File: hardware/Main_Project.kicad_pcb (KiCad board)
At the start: 2 copper layers, 246.8 x 135.9 mm, 64 parts, among them J1 Motors_R, J10 BBBBBBBONUSROUND, J11 Power_Distro, J12 Power_Distro, J13 Power_Distro, J14 Power_Distro, J15 Color_Sensor, J16 Color_Sensor, J2 Motors_L, J3 Power_Outputs, J4 Motor_Control, J5 Motor_Power, J6 Motor_Power, J7 Motor_Control, J8 Color_Sensor, J9 Magnet?, U1 L7805, U2 L298N

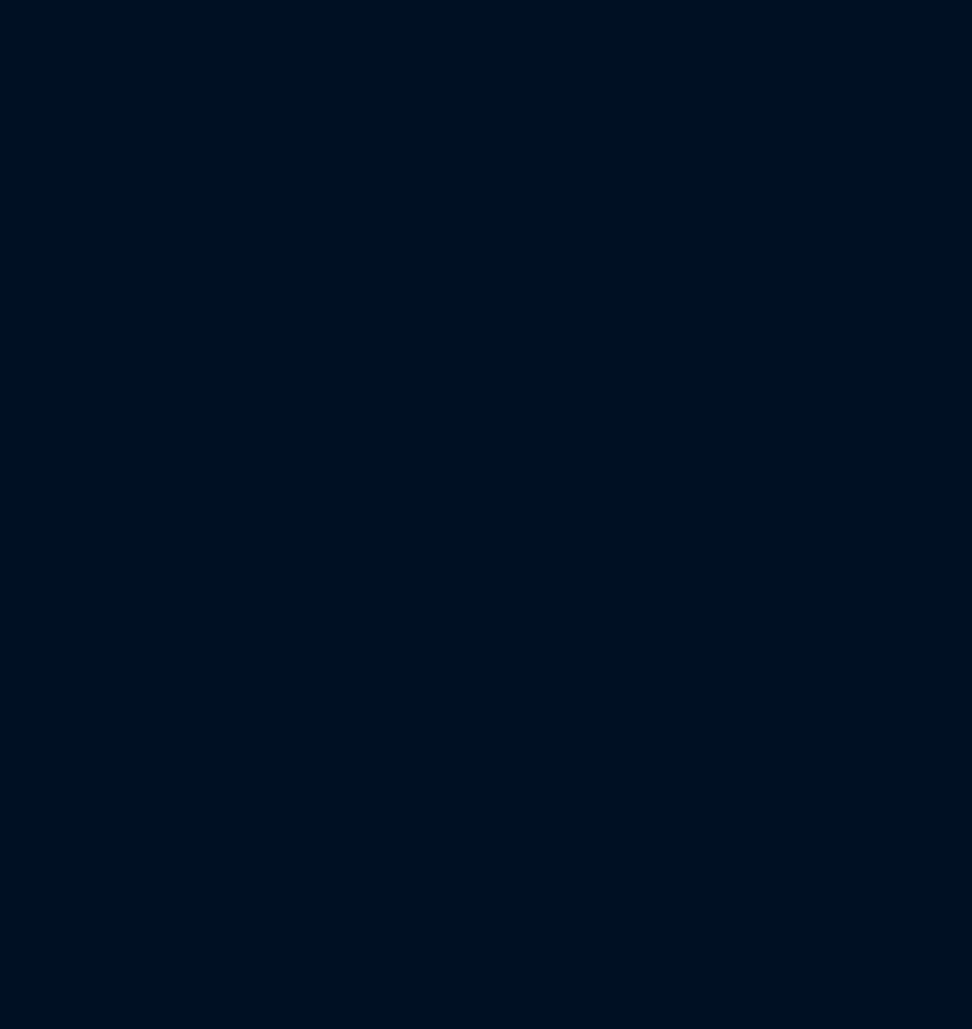
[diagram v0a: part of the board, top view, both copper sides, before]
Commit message: Magnet board
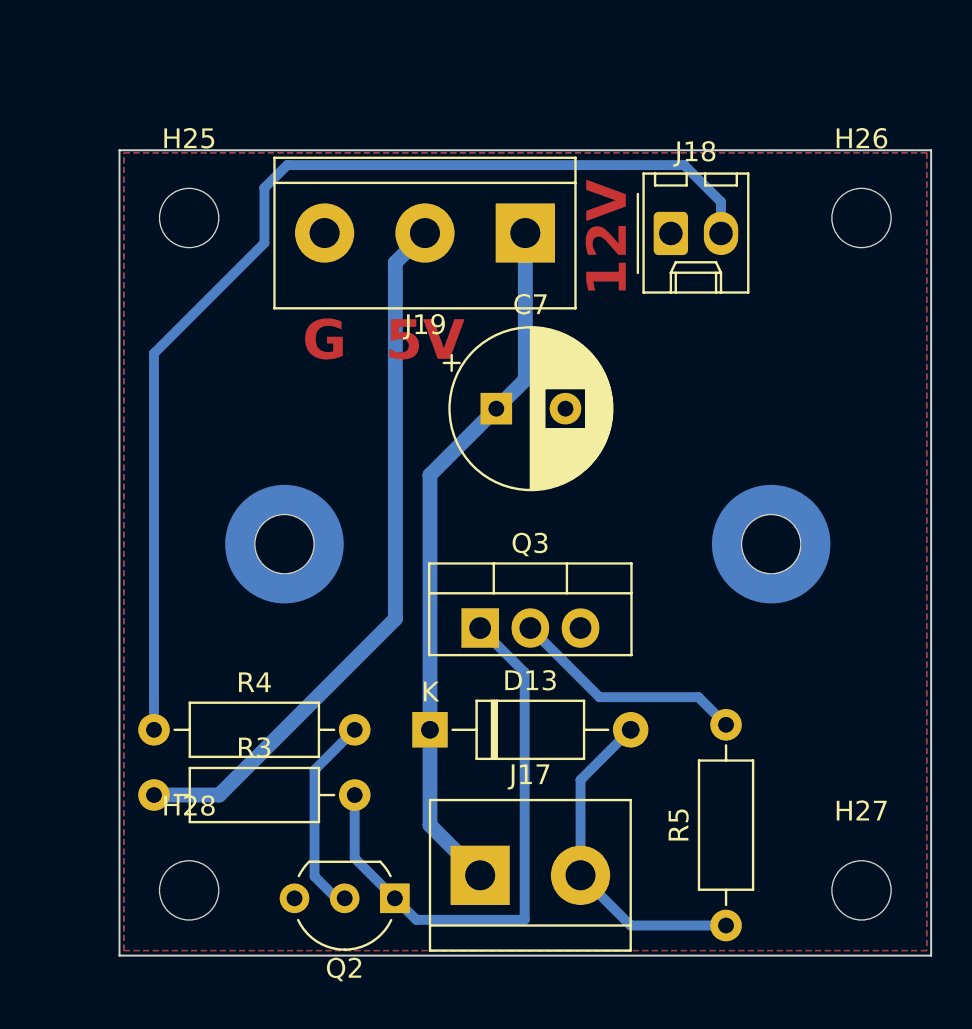
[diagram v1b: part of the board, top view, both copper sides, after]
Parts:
- added C7: 4.7uF, Capacitor_THT:CP_Radial_D8.0mm_P3.50mm, F.Cu at (252.3, 135.9)
- added D13: 1N4004, Diode_THT:D_A-405_P10.16mm_Horizontal, F.Cu at (248.9, 152.1)
- added H23: HeatsinkMounting, new_winterbloom:M3_Heatsink_Mounting, F.Cu at (266.2, 142.7)
- added H24: HeatsinkMounting, new_winterbloom:M3_Heatsink_Mounting, F.Cu at (241.6, 142.7)
- added H25: MountingHole, MountingHole:MountingHole_3mm, F.Cu at (236.7, 126.2)
- added H26: MountingHole, MountingHole:MountingHole_3mm, F.Cu at (270.8, 126.2)
- added H27: MountingHole, MountingHole:MountingHole_3mm, F.Cu at (270.8, 160.3)
- added H28: MountingHole, MountingHole:MountingHole_3mm, F.Cu at (236.7, 160.3)
- added J17: Magnet, TerminalBlock:TerminalBlock_bornier-2_P5.08mm, F.Cu at (251.5, 159.5)
- added J18: FRDM input, Connector_Molex:Molex_KK-254_AE-6410-02A_1x02_P2.54mm_Vertical, F.Cu at (261.1, 127.0)
- added J19: Magnet_Power, TerminalBlock:TerminalBlock_bornier-3_P5.08mm, F.Cu at (253.7, 127.0)
- added Q2: BC547, Package_TO_SOT_THT:TO-92_Inline_Wide, F.Cu at (247.1, 160.7)
- added Q3: IRF540N, Package_TO_SOT_THT:TO-220-3_Vertical, F.Cu at (251.5, 147.0)
- added R3: 10k, Resistor_THT:R_Axial_DIN0207_L6.3mm_D2.5mm_P10.16mm_Horizontal, F.Cu at (235.0, 155.4)
- added R4: 1k, Resistor_THT:R_Axial_DIN0207_L6.3mm_D2.5mm_P10.16mm_Horizontal, F.Cu at (235.0, 152.1)
- added R5: Current_Limit, Resistor_THT:R_Axial_DIN0207_L6.3mm_D2.5mm_P10.16mm_Horizontal, F.Cu at (263.9, 162.1)
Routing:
- net Net-(J18-Pin_2): track 0.00 -> 55.7 mm
- net +5V: track 203.9 -> 240.0 mm
- net +12V: track 285.9 -> 321.4 mm
- net Net-(Q2-C): track 0.00 -> 28.8 mm
- net Net-(D13-A): track 0.00 -> 16.8 mm
- net Net-(Q3-D): track 0.00 -> 11.9 mm
- net Net-(Q2-B): track 0.00 -> 10.2 mm
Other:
- board size 246.8 x 135.9 mm -> 254.1 x 139.2 mm
